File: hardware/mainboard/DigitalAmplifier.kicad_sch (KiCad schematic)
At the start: 54 parts, among them J10 FFC2B35-10-T, J12 Conn_01x02, J2 Conn_01x02, J3 Conn_01x02, J4 Conn_01x02, J5 USB4215-03-A_REVA, J6 Conn_01x02, J7 43045-0414, J9 Conn_01x02, U1 ORJ-3__FCR6842032R_

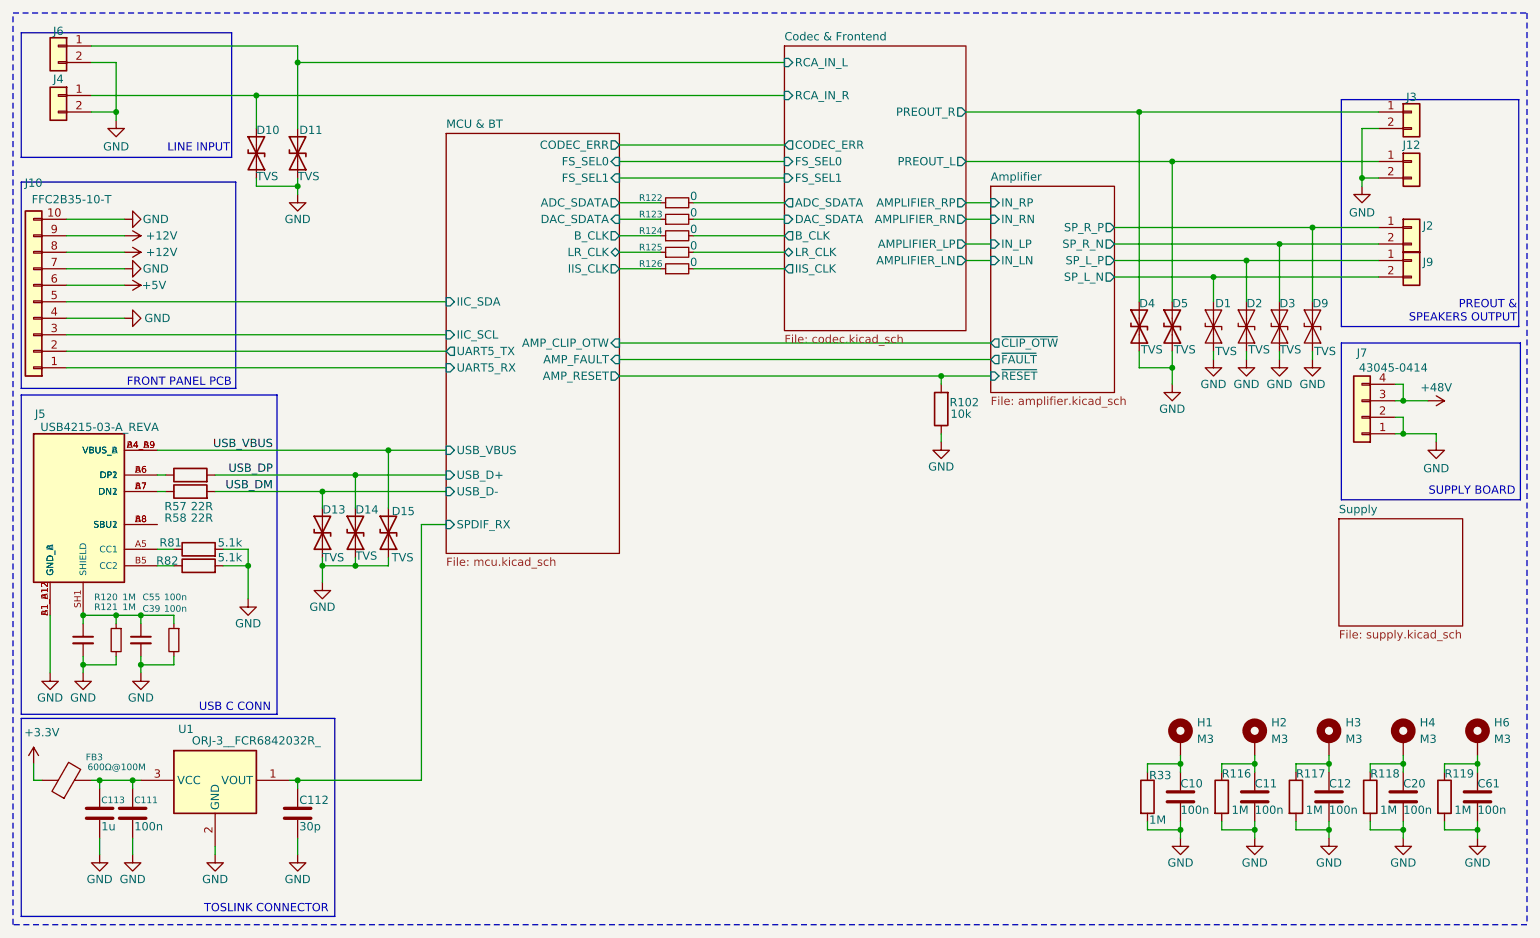
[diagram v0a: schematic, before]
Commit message: Prepare PCB for production
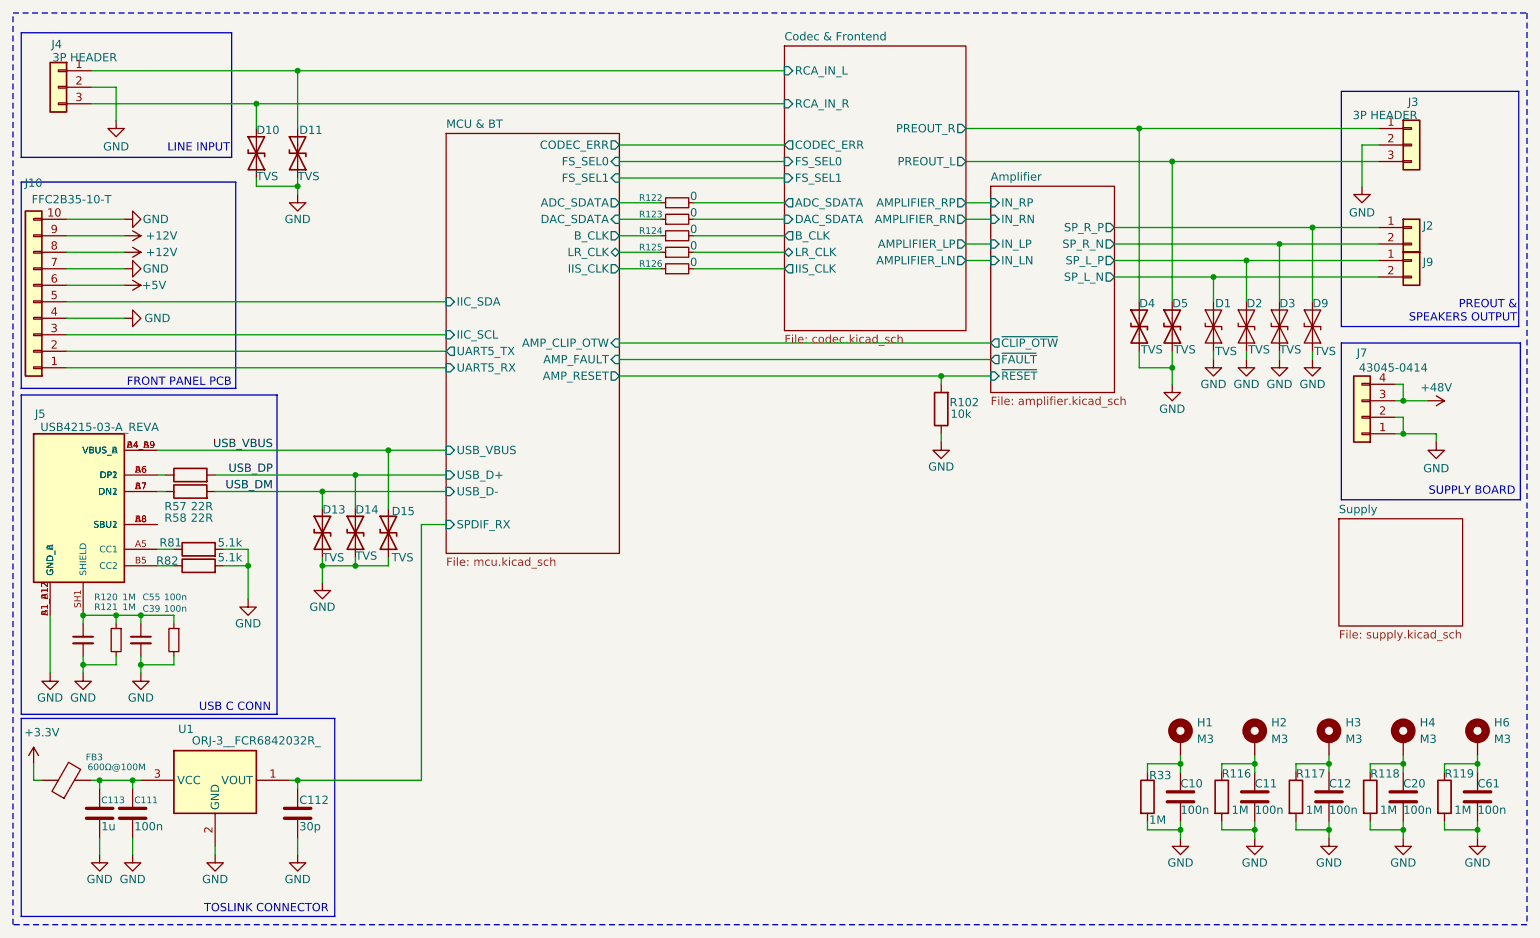
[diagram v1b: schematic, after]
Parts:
- removed J12, J3, J4, J6: Conn_01x02, digital_amp:RF219AT0050G, symbol Connector_Generic:Conn_01x02
- added J3, J4: 3P HEADER, Connector_JST:JST_PH_B3B-PH-K_1x03_P2.00mm_Vertical, symbol Connector_Generic:Conn_01x03
- C10, C11, C111, C12, C20, C39, C55, C61: Manufacturer_Part_Number (none) -> 0603B104K500CT
- C112: Manufacturer_Part_Number (none) -> C0603C300J5GACTU
- C113: Manufacturer_Part_Number (none) -> CL10A105KB8NNNC
- H1, H2, H3, H4, H6: Manufacturer_Part_Number (none) -> 9774040360R
- J10: Manufacturer_Part_Number (none) -> FFC2B3510T
- J2, J9: Manufacturer_Part_Number (none) -> 43650-0215
- J5: Manufacturer_Part_Number (none) -> GCT_USB4215-03-A_REVA
- J7: Manufacturer_Part_Number (none) -> 43045-04YY_121314
- R102: Manufacturer_Part_Number (none) -> RC0603JR-0710KL
- R116, R117, R118, R119, R120, R121, R33: Manufacturer_Part_Number (none) -> RC0603JR-071ML
- R122, R123, R124, R125, R126: Manufacturer_Part_Number (none) -> RC0402JR-070RL
- R57, R58: Manufacturer_Part_Number (none) -> WR06X220 JTL
- R81, R82: Manufacturer_Part_Number (none) -> WR06X5101FTL
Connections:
- net Codec & Frontend/PREOUT_L: now also J3.3 (Pin_3)
- net Codec & Frontend/PREOUT_R: now also J3.1 (Pin_1)
- net Codec & Frontend/RCA_IN_L: now also J4.1 (Pin_1)
- net Codec & Frontend/RCA_IN_R: now also J4.3 (Pin_3)
- net GND: now also J3.2 (Pin_2), J4.2 (Pin_2)
